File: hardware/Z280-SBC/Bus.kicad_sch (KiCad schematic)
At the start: 6 parts, among them J4 ATF-JTAG-10, J5 COUNTER1, J6 ADBUS, J7 SIGBUS, J8 IE/OE, U10 ATF1504AS-xJx44

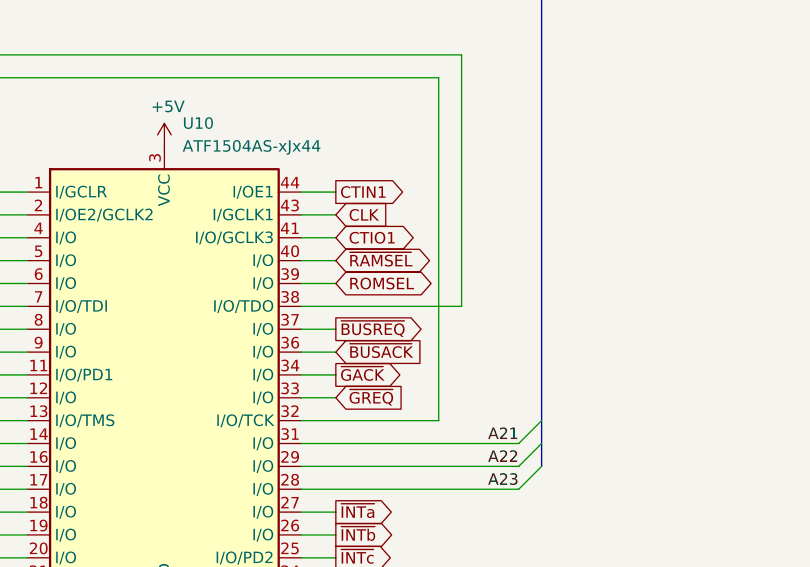
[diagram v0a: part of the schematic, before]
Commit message: Rev1 - All connections completed
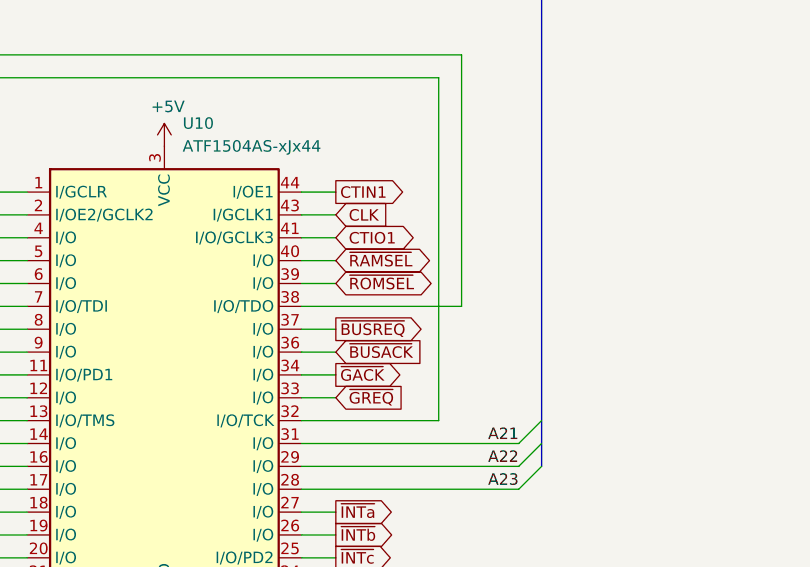
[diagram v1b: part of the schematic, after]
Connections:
- net ROMSEL is gone; now on net ~{ROMSEL}: U10.39 (I/O)
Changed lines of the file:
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@@
     )
   )
-  (global_label "ROMSEL" (shape bidirectional) (at 128.27 60.96 0) (fields_autoplaced)
+  (global_label "~{ROMSEL}" (shape bidirectional) (at 128.27 60.96 0) (fields_autoplaced)
     (effects (font (size 1.27 1.27)) (justify left))
     (property "Intersheet References" "${INTERSHEET_REFS}" (id 0) (at 138.1217 60.8806 0)
